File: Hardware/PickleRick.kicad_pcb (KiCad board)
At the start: 4 copper layers, 100 x 37 mm, 205 parts, among them IC1 TPS259830ONRGER, J1 RBUS, J10 Conn_Coaxial, J11 Conn_Coaxial, J12 Conn_01x03_Male, J13 Conn_01x03_Pin, J14 Conn_01x07_Socket, J2 Conn_01x02_Male, J3 ST1W008S4TR2000, J4 Conn_01x03_Pin, J5 USB_C_Receptacle_USB2.0, J6 Screw_Terminal_01x08, J7 Conn_01x05_Male, J8 DeployLipo, J9 UCLipo, Q1 PMV20ENR, Q10 DMP3099L, Q11 SQS141ELNW-T1_GE3, Q12 SQS141ELNW-T1_GE3, Q2 BUK9M11-40EX, Q3 BUK9M11-40EX, Q4 BUK9M11-40EX, Q5 BUK9M11-40EX, Q8 DMP3099L, Q9 DMP3099L, U1 ESP32-S3, U10 LTC4412xS6, U11 MP28167GQ-A-Z, U14 LTC4412xS6, U16 SC4215, U17 LTC4412xS6, U19 MAX-M10S, U2 DPS368, U20 SN65HVD230, U21 RFM95W-868S2, U22 LTC4412xS6, U3 LTV-247, U4 PCA9534RGVR, U5 PCA9685BS, U6 H3LIS331DLTR, U7 ICM-20608-G, U8 MMC5983MA, U9 LTC4412xS6, Y1 R940000171

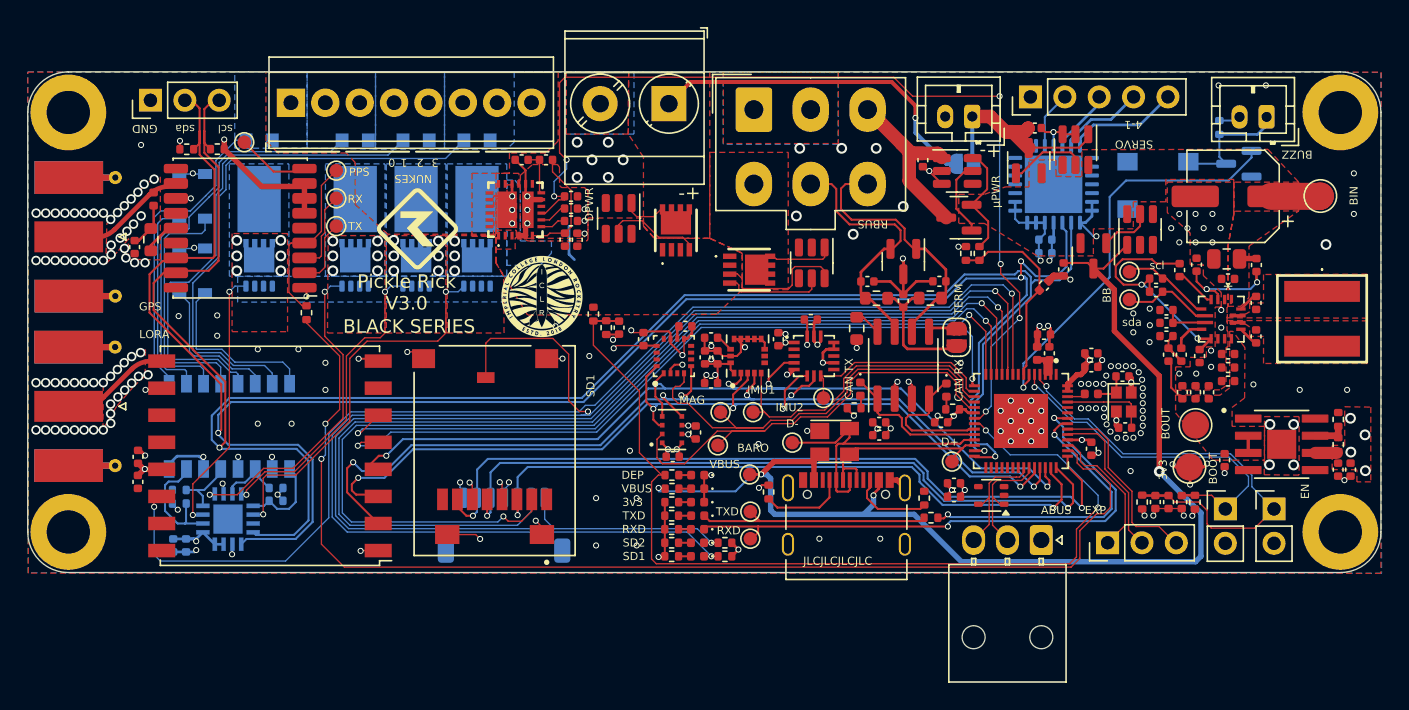
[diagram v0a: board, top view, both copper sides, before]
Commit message: hardware update
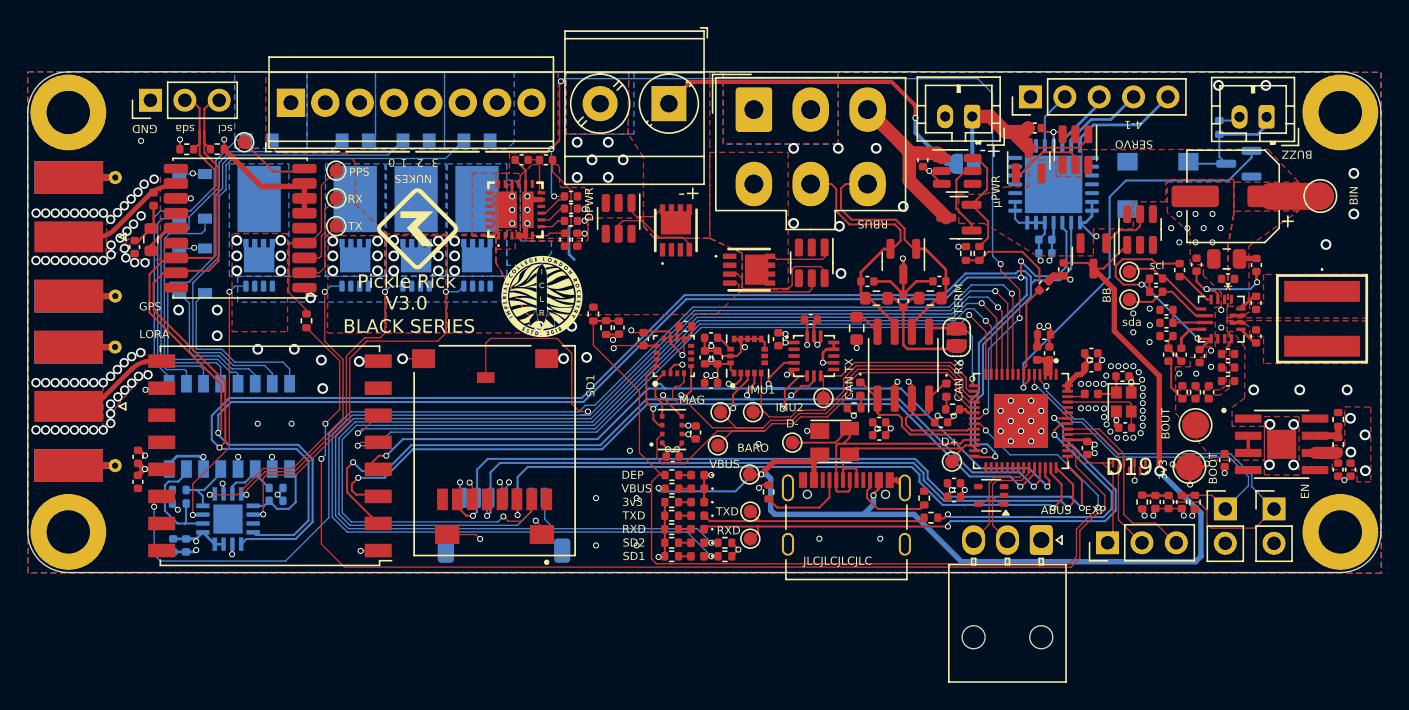
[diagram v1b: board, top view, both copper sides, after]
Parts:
- added D19: RCLAMP3346PQTNT, iclr-hw:RCLAMP3346PQTNT, F.Cu at (181.4, 89.2)
- moved R8 0.60 mm to (120.6, 78.4)
- moved C10 0.30 mm to (178.3, 87.8)
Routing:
- net GND: track 110.5 -> 113.0 mm, vias 230 -> 231
- net /JTAG_MTCK: track 86.4 -> 84.8 mm
- net +3V3: track 70.4 -> 71.2 mm
- net /DepCurrent: track 71.3 -> 70.8 mm
